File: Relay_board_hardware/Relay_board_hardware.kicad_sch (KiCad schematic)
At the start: 16 parts, among them IC1 BTS3800SL, Q1 IRF740ASPBF, U1 MCP6497T-E/SN

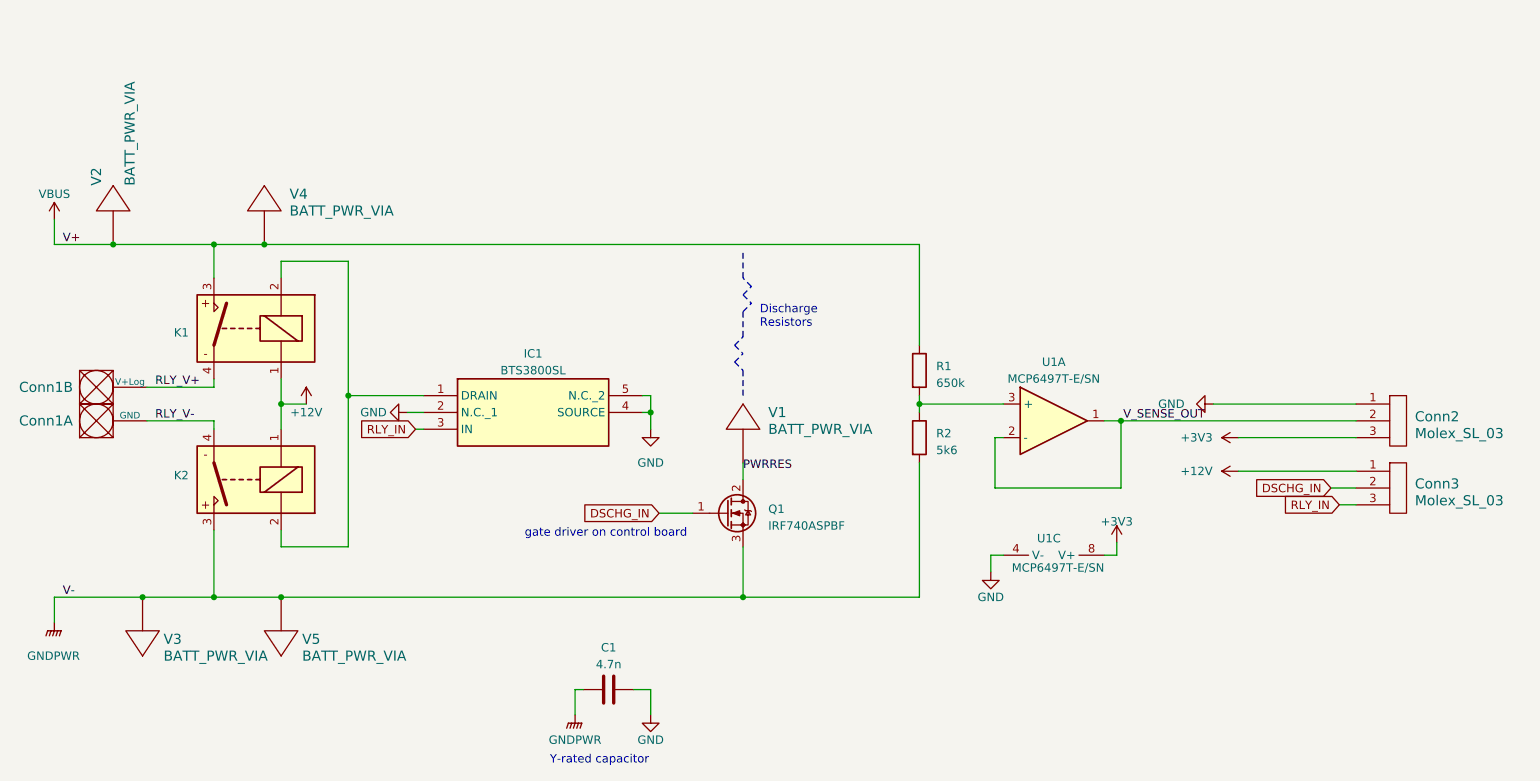
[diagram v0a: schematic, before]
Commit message: R2 edits
gerbs generated
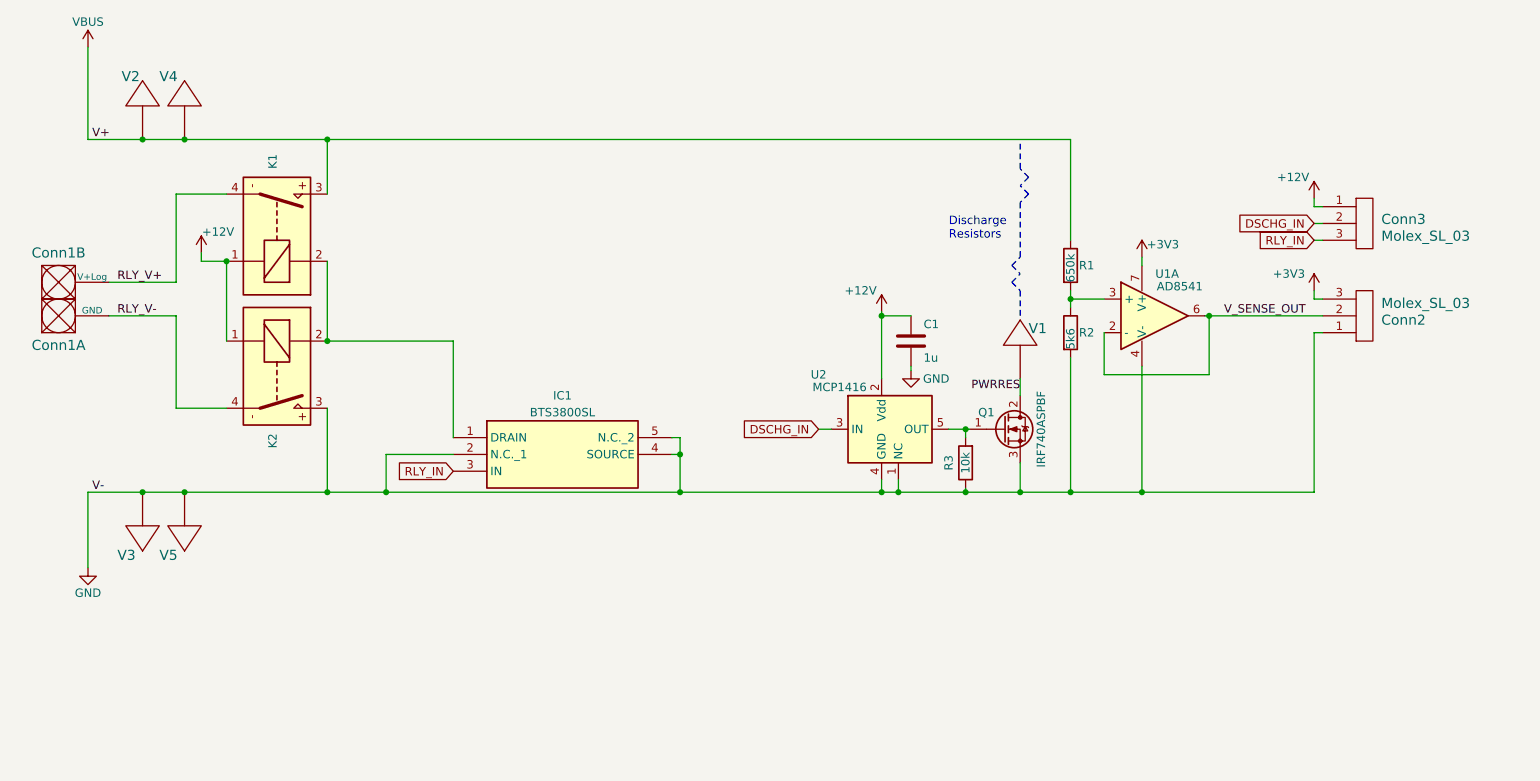
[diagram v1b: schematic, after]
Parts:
- added R3: 10k, Resistor_SMD:R_0603_1608Metric_Pad0.98x0.95mm_HandSolder, symbol Device:R
- added U2: MCP1416, Package_TO_SOT_SMD:SOT-23-5, symbol Driver_FET:MCP1416
- C1: value 4.7n -> 1u; footprint Capacitor_THT:C_Rect_L13.0mm_W5.0mm_P10.00mm_FKS3_FKP3_MKS4 -> Capacitor_SMD:C_0603_1608Metric_Pad1.08x0.95mm_HandSolder; Price 0.46 -> (none)
- U1: value MCP6497T-E/SN -> AD8541
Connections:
- net +12V: now also C1.1, U2.2 (Vdd)
- net +3V3: now also U1.7 (V+); no longer U1.8 (V+)
- net DSCHG_IN: now also U2.3 (IN); no longer Q1.1 (G)
- net GND: now also K2.3, Q1.3 (S), R2.2, V3.1, V5.1, R3.1, U2.1 (NC), U2.4 (GND)
- net V_SENSE_OUT: now also U1.6; no longer U1.1
- removed net GNDPWR: C1.1, K2.3, Q1.3 (S), R2.2, V3.1, V5.1
- new net: Q1.1 (G), R3.2, U2.5 (OUT)
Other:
- note removed: "Y-rated capacitor"
- note removed: "gate driver on control board"
- moved on the sheet: Conn1A, Conn1B, Conn2, Conn3, IC1, K1, K2, Q1, R1, R2, U1A, V1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
